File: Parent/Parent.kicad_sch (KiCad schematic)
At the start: 0 parts

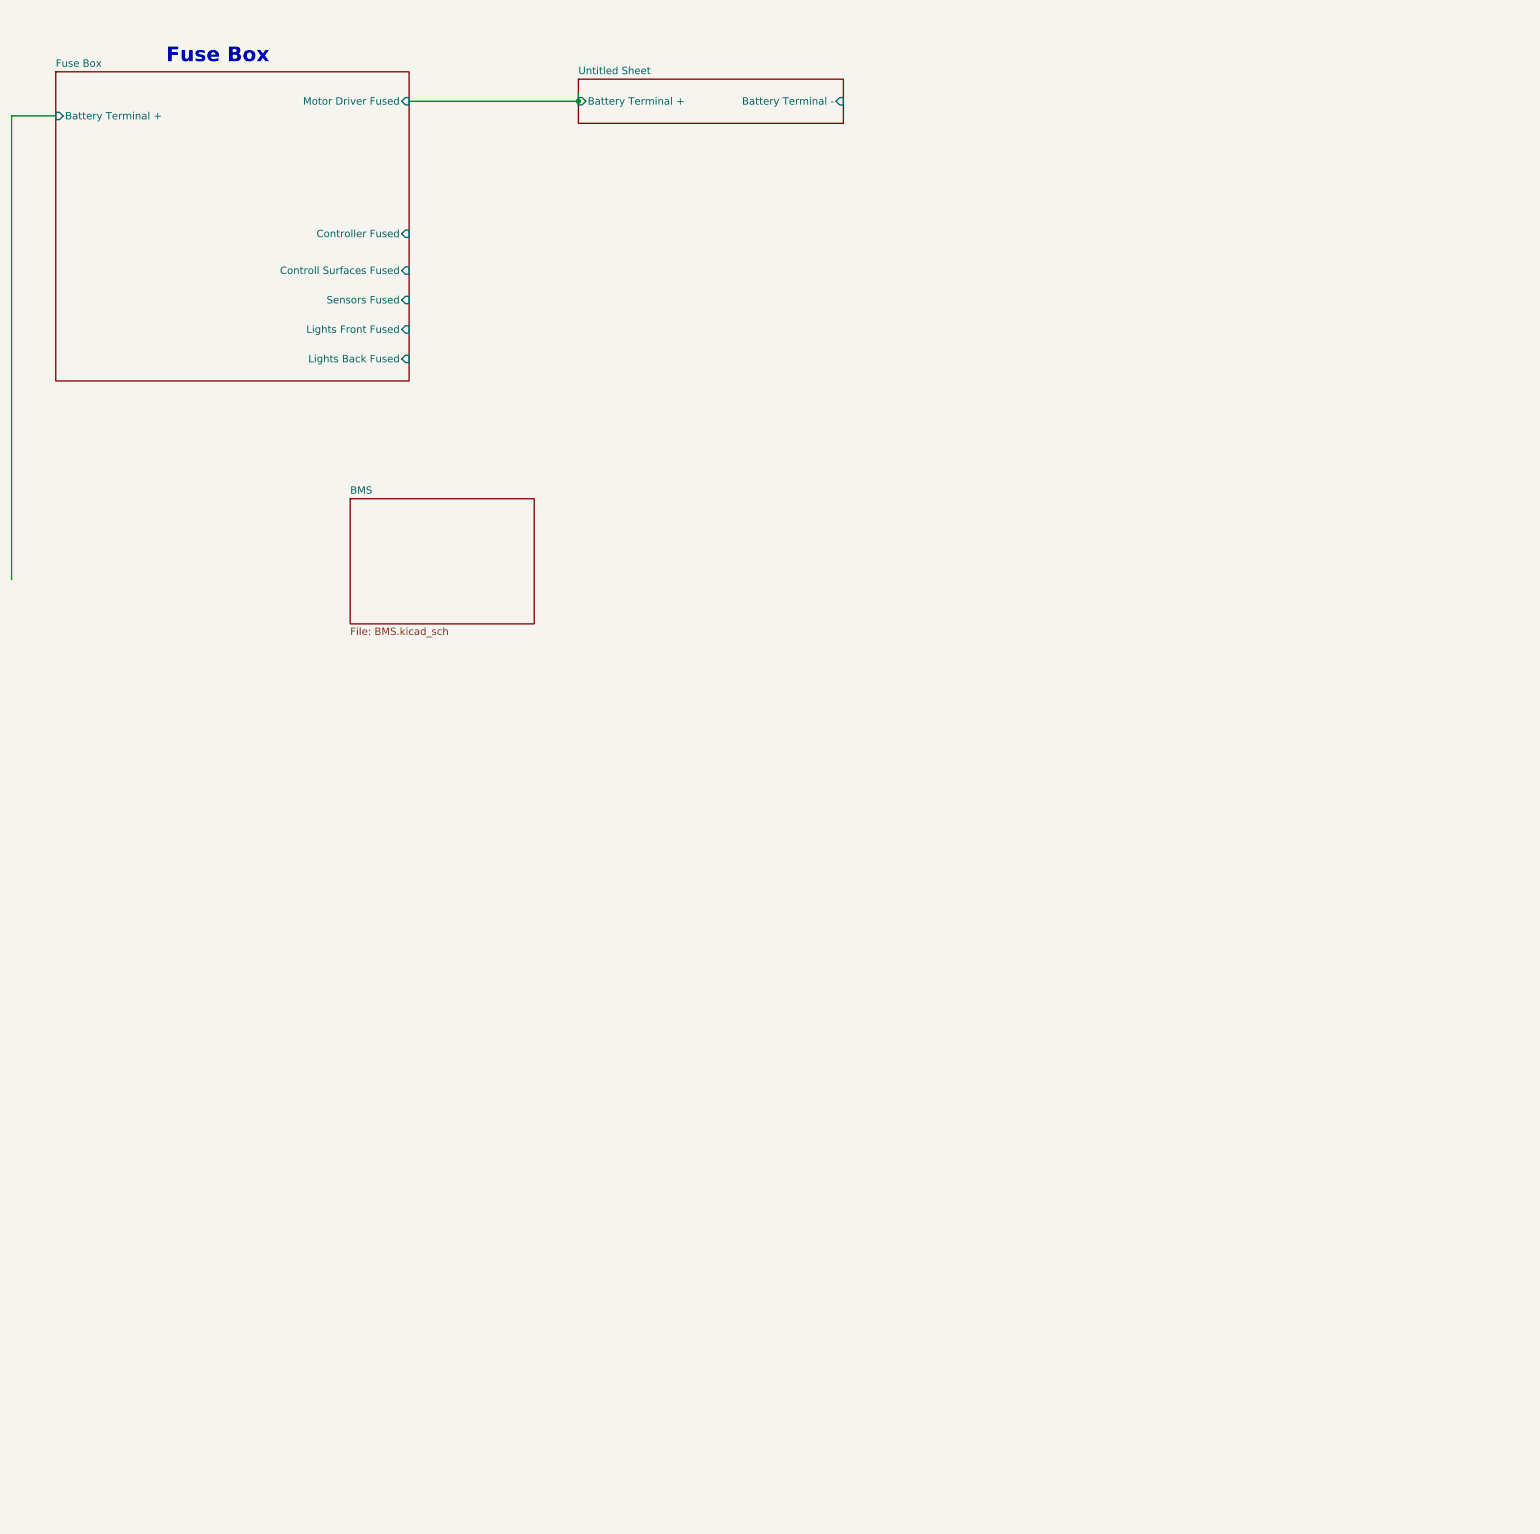
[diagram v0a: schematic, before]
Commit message: Worked on Parent - Move Workspace to cloud
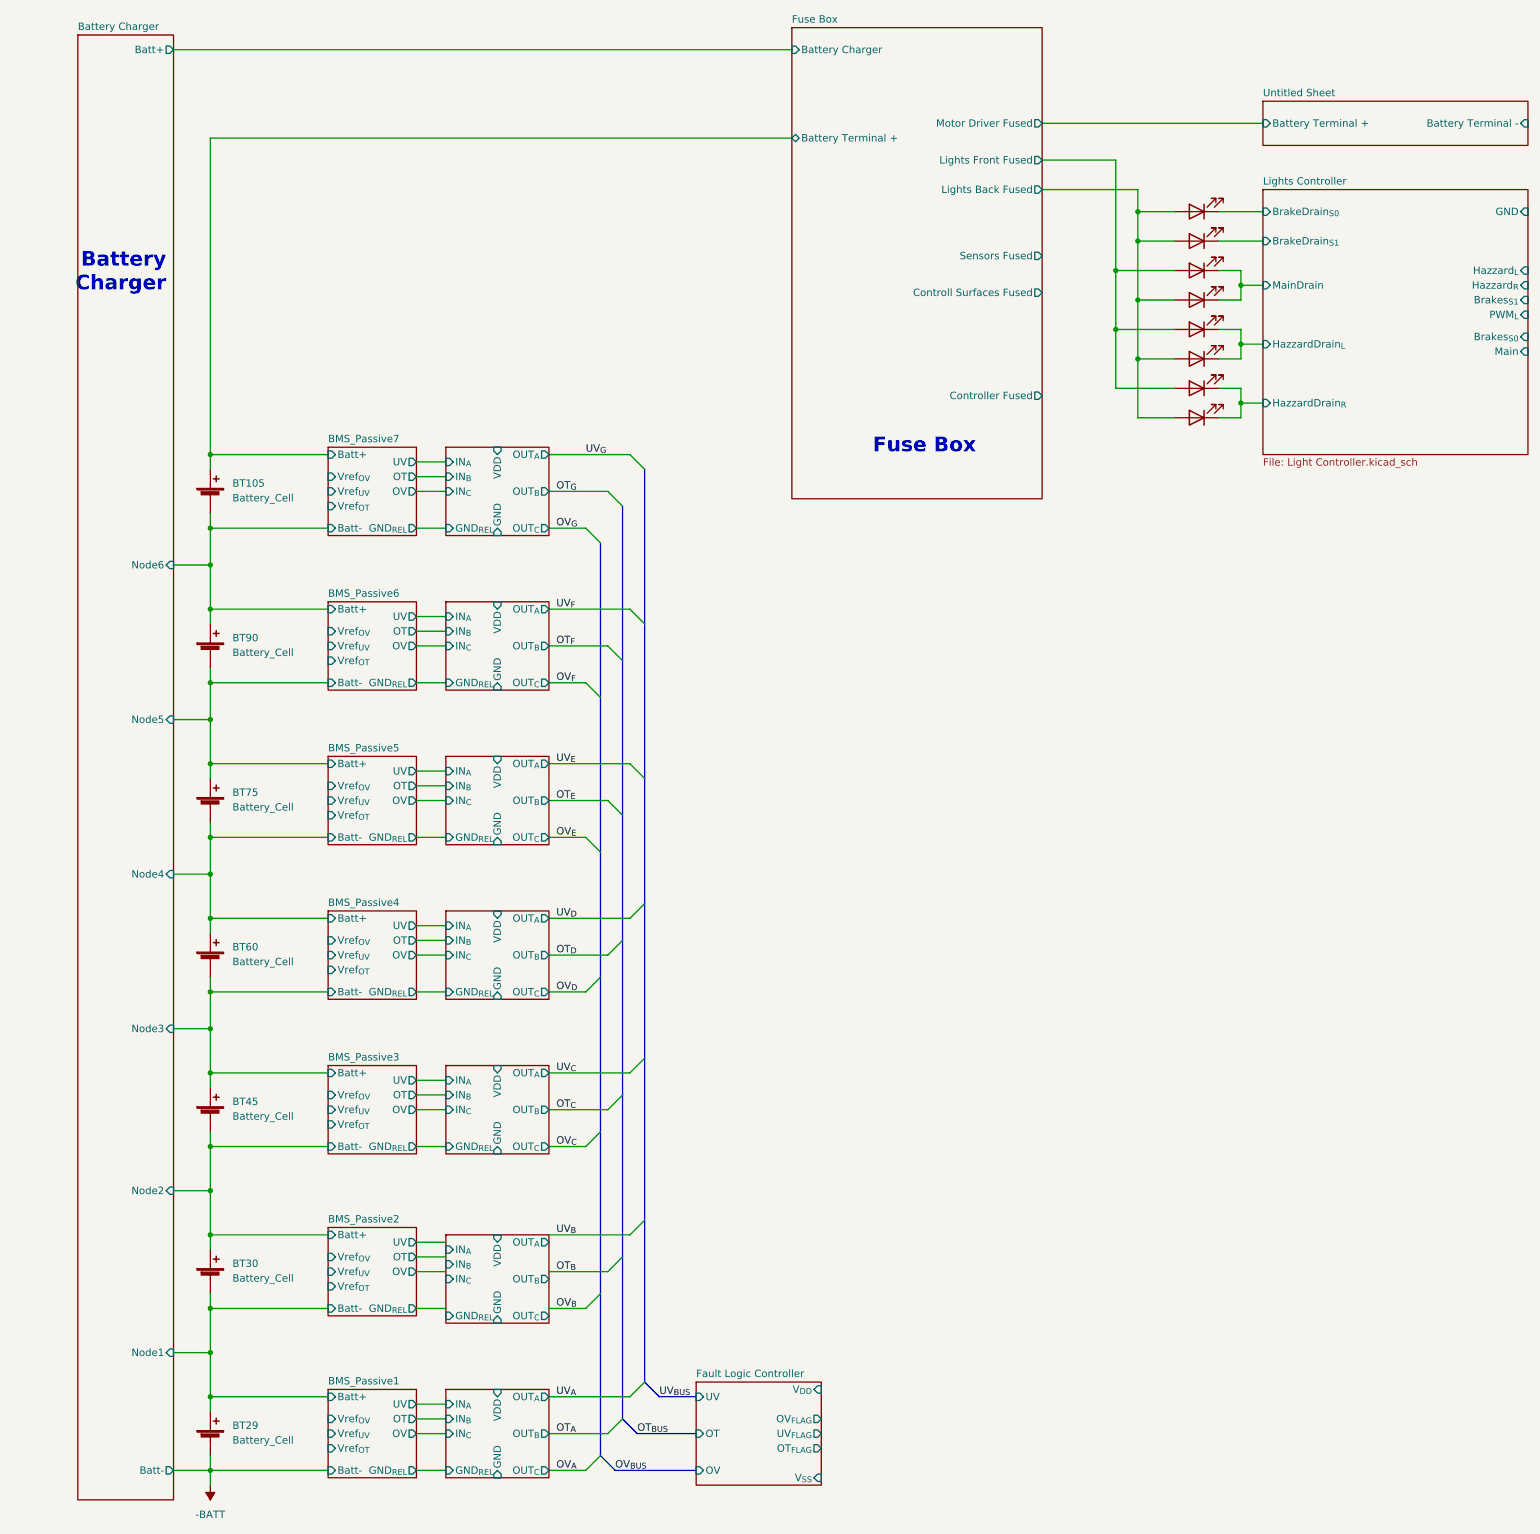
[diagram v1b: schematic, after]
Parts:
- added BT105, BT29, BT30, BT45, BT60, BT75, BT90: Battery_Cell, symbol Device:Battery_Cell
- added D1, D2, D3, D4, D5, D6, D7, D8: LED, symbol Device:LED
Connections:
- net Fuse Box/Lights Back Fused: now also D1.2 (A), D2.2 (A), D4.2 (A), D6.2 (A), D8.2 (A)
- net Fuse Box/Lights Front Fused: now also D3.2 (A), D5.2 (A), D7.2 (A)
- new net -BATT: BT29.2 (-)
- new net BMS_Passive1/Batt+: BT29.1 (+), BT30.2 (-)
- new net BMS_Passive2/Batt+: BT30.1 (+), BT45.2 (-)
- new net BMS_Passive3/Batt+: BT45.1 (+), BT60.2 (-)
- new net BMS_Passive4/Batt+: BT60.1 (+), BT75.2 (-)
- new net BMS_Passive5/Batt+: BT75.1 (+), BT90.2 (-)
- new net BMS_Passive6/Batt+: BT105.2 (-), BT90.1 (+)
- new net BMS_Passive7/Batt+: BT105.1 (+)
- new net Lights Controller/BrakeDrain_{S0}: D1.1 (K)
- new net Lights Controller/BrakeDrain_{S1}: D2.1 (K)
- new net Lights Controller/HazzardDrain_{L}: D5.1 (K), D6.1 (K)
- new net Lights Controller/HazzardDrain_{R}: D7.1 (K), D8.1 (K)
- new net Lights Controller/MainDrain: D3.1 (K), D4.1 (K)
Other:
- removed sheet BMS
- added sheet BMS_Passive1 (BMS_Passive.kicad_sch)
- added sheet BMS_Passive2 (BMS_Passive.kicad_sch)
- added sheet BMS_Passive3 (BMS_Passive.kicad_sch)
- added sheet BMS_Passive4 (BMS_Passive.kicad_sch)
- added sheet BMS_Passive5 (BMS_Passive.kicad_sch)
- added sheet BMS_Passive6 (BMS_Passive.kicad_sch)
- added sheet BMS_Passive7 (BMS_Passive.kicad_sch)
- added sheet Battery Charger (BatteryCharger.kicad_sch)
- added sheet Fault Logic Controller (FaultLogicController.kicad_sch)
- added sheet Level Translator1 (LevelTranslator.kicad_sch)
- added sheet Level Translator2 (LevelTranslator.kicad_sch)
- added sheet Level Translator3 (LevelTranslator.kicad_sch)
- added sheet Level Translator4 (LevelTranslator.kicad_sch)
- added sheet Level Translator5 (LevelTranslator.kicad_sch)
- added sheet Level Translator6 (LevelTranslator.kicad_sch)
- added sheet Level Translator7 (LevelTranslator.kicad_sch)
- added sheet Lights Controller (Light Controller.kicad_sch)
- sheet Fuse Box ports: added Battery Charger ; removed none
- note added: "Battery Charger"
